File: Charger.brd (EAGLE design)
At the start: 25.1 x 25.4 mm, 11 parts, among them IC1 MAX1044

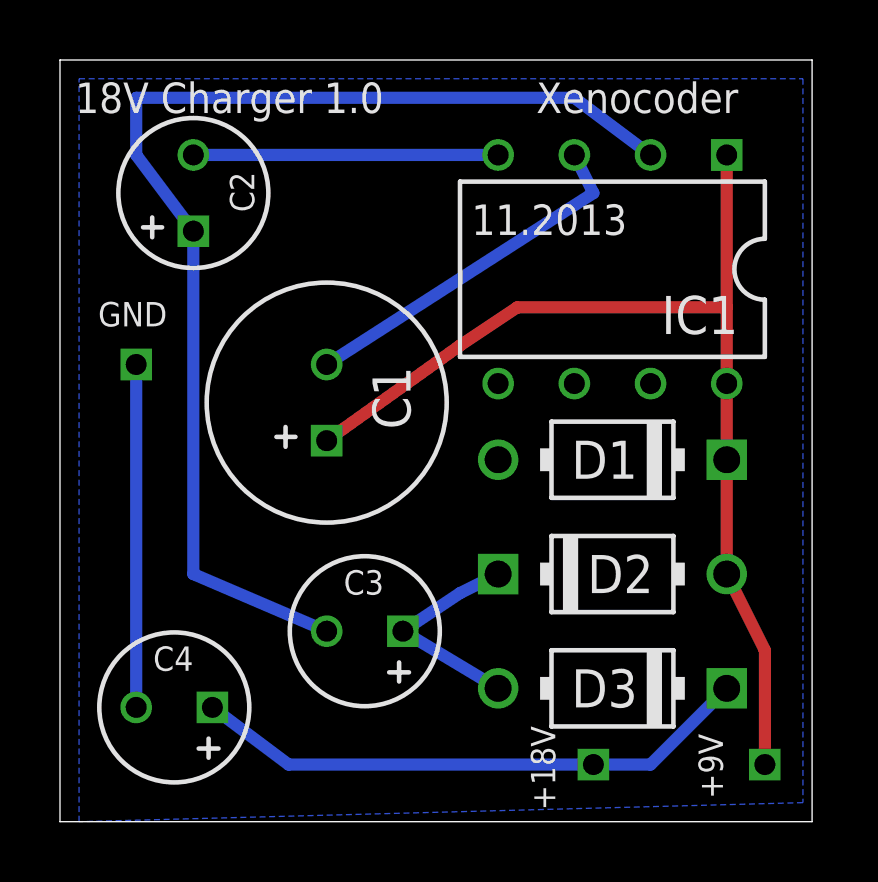
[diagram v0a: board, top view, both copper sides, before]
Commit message: Changes in schematic and board to v1.1
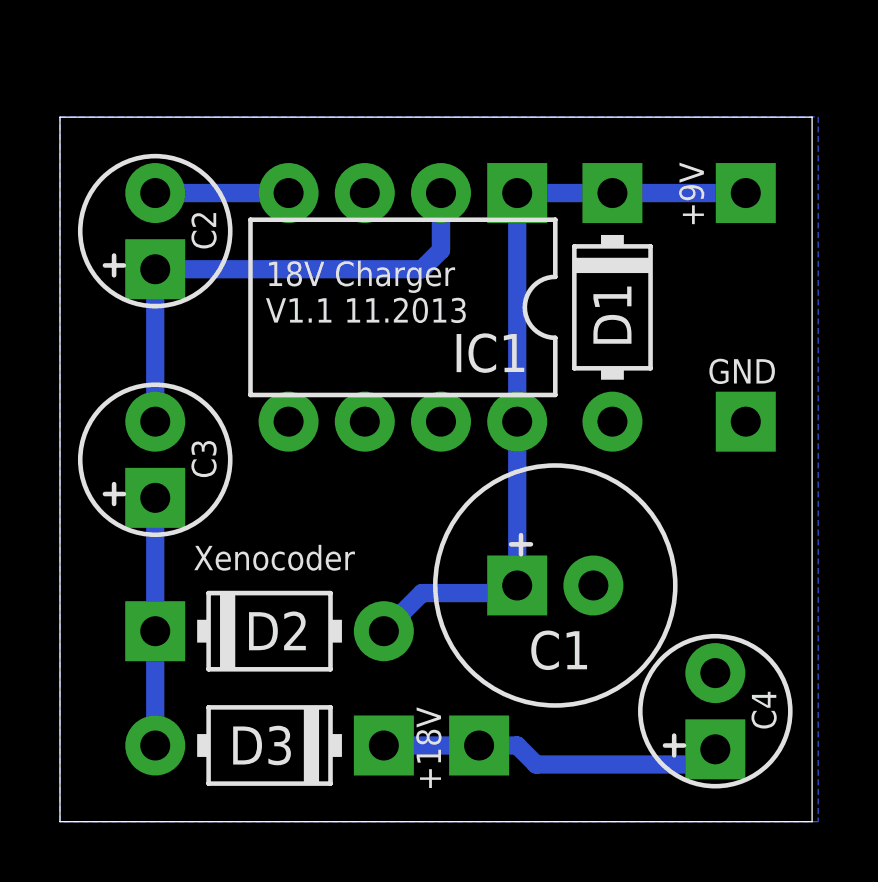
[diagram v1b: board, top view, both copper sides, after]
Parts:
- +18V, +9V, GND: device gm-supply:SQUARE -> mb_supply:SQUARE
- C1: device gm-caps-electro-pol:080_035_1 -> mb_caps-electro:080_035_1
- C2, C3, C4: device gm-caps-electro-pol:050_020_1 -> mb_caps-electro:050_020_1
- D1, D2, D3: device gm-diodes:DO41-3 -> mb_diodes:DO41-3
- IC1: device gm-ics:DIL08 -> mb_ics:DIL08
- moved GND 20.4 mm to (22.9, 13.3)
- moved +9V 19.1 mm to (22.9, 21.0)
- moved C4 18.0 mm to (21.8, 3.68), turned to 90 degrees
- moved D2 11.6 mm to (6.99, 6.35)
- moved D3 11.6 mm to (6.99, 2.54)
- moved C1 9.76 mm to (16.5, 7.87), turned to 0 degrees
- moved C3 9.03 mm to (3.17, 12.1), turned to 90 degrees
- moved IC1 7.10 mm to (11.4, 17.1)
- moved D1 5.08 mm to (18.4, 17.1), turned to 270 degrees
- moved +18V 3.86 mm to (14.0, 2.54)
- moved C2 1.80 mm to (3.17, 19.7)
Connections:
- removed net N$1: C1.-, IC1.3
- net GND: now also C1.-, IC1.3
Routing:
- net N$3: track 39.1 -> 16.8 mm
- net N$1: track 12.0 -> 0.00 mm
- net GND: track 11.4 -> 0.00 mm
- net +9V: track 35.4 -> 25.8 mm
- net +18V: track 18.8 -> 11.5 mm
- net N$2: track 10.2 -> 4.45 mm
- net N$4: track 7.41 -> 8.25 mm
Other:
- board size 25.1 x 25.4 mm -> 25.1 x 23.5 mm
- board text added: "18V Charger V1.1 11.2013"
- board text removed: "11.2013"
- board text removed: "18V Charger 1.0"
